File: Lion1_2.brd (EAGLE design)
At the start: 100 x 85.7 mm, 71 parts, among them IC1 MCP4822, IC2 MCP4822, IC3 MCP4822, IC4 REG1117, U7 2564-, U8 2564-

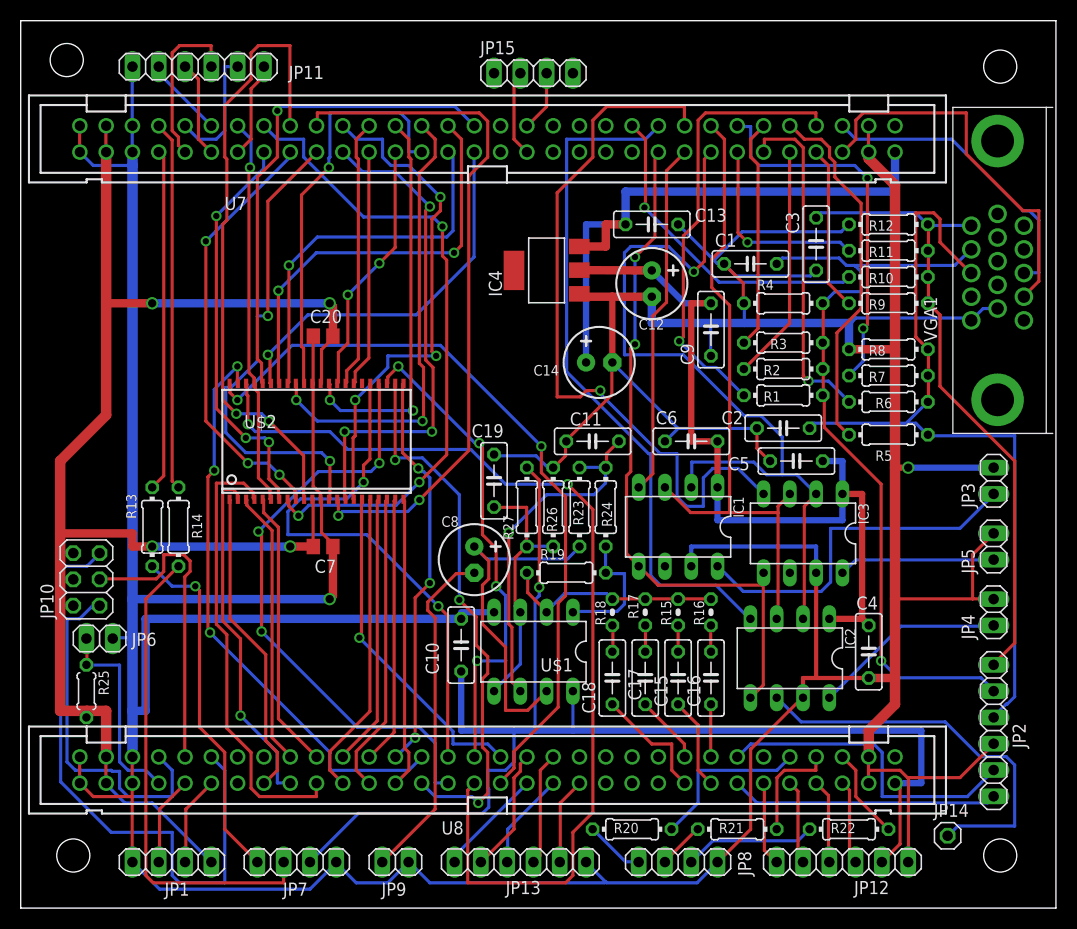
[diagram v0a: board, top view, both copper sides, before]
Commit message: v2
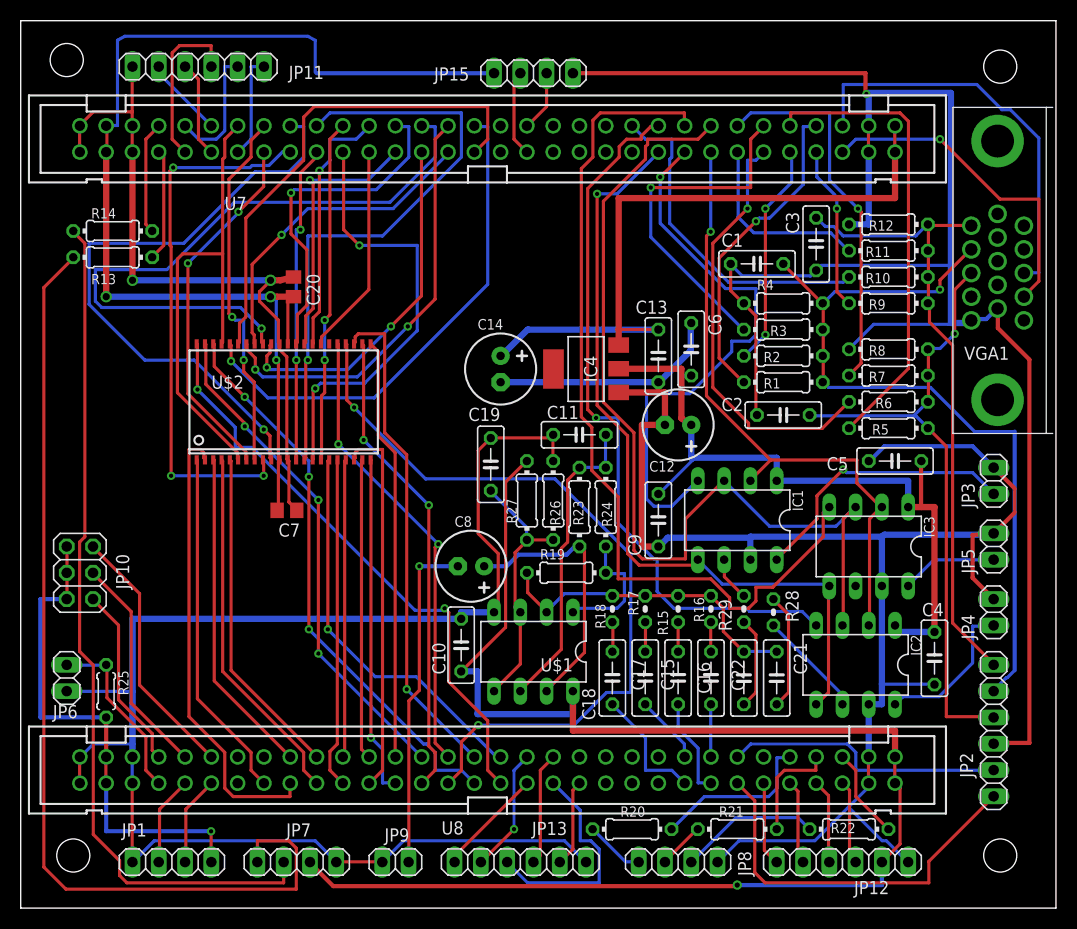
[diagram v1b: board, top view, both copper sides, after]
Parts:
- removed JP14: (no value), pinhead:1X01
- added C21, C22: 4.7uf, rcl:C050-025X075
- added R28, R29: (no value), SmartPrj:0204V
- C13: value 100nf -> (none)
- moved R14 29.3 mm to (8.89, 65.4), turned to 180 degrees
- moved R13 26.3 mm to (8.89, 62.9), turned to 180 degrees
- moved C9 19.1 mm to (61.6, 37.5)
- moved C12 13.9 mm to (63.5, 46.7), turned to 180 degrees
- moved C13 12.7 mm to (61.6, 53.3), turned to 90 degrees
- moved IC4 10.3 mm to (54.6, 52.1)
- moved C14 9.55 mm to (46.4, 52.1), turned to 270 degrees
- moved C5 9.52 mm to (84.5, 43.2)
- moved C6 8.89 mm to (64.8, 54.0), turned to 270 degrees
- moved IC3 6.48 mm to (81.9, 34.9)
- moved C4 6.38 mm to (88.3, 24.1)
- moved IC2 6.38 mm to (80.6, 23.5)
- moved IC1 5.75 mm to (69.2, 37.5)
- moved C20 5.55 mm to (26.4, 60.0), turned to 270 degrees
- moved U$2 4.96 mm to (25.4, 48.9)
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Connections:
- net N$24 renamed TX2
- net N$85 renamed RX2
- removed net 3V3: C20.2, C7.2, JP1.4, JP10.2, JP10.4, JP10.6, R25.2, U$2.11, U$2.33, U7.3, U7.4, U8.3, U8.4
- removed net GND: C1.1, C10.1, C11.2, C12.-, C13.1, C14.-, C19.1, C2.1, C20.1, C3.1, C4.1, C5.1, C6.1, C7.1, C9.1, IC1.7, IC2.7, IC3.7, IC4.1, JP1.1, JP11.1, JP12.1, JP13.1, JP2.4, JP3.2, JP4.2, JP5.2, JP6.2, JP7.4, JP8.4, JP9.2, R12.1, R26.1, R4.1, R8.1, U$1.4, U$2.12, U$2.34, U7.1, U7.2, U7.5, U7.6, U7.61, U7.62, U8.1, U8.2, U8.5, U8.6, U8.61, U8.62, VGA1.10, VGA1.5
- removed net N$70: U8.64
- new net 3V3_7: C20.2, C7.2, JP15.1, U$2.11, U$2.33, U7.3, U7.4
- new net 3V3_8: JP1.4, JP10.2, JP10.4, JP10.6, R25.2, U8.3, U8.4
- new net ADD: C21.1, C22.1, R15.2, R16.2, R17.2, R18.2, R19.1, U$1.2
- new net GND7_61: C1.1, C2.1, C3.1, JP15.4, JP2.4, R12.1, R4.1, R8.1, U7.61, U7.62, VGA1.10, VGA1.5
- new net GND8_1: C10.1, C11.2, C19.1, JP1.1, JP13.1, JP6.2, JP7.4, JP9.2, R26.1, U$1.4, U8.1, U8.2, U8.5, U8.6
- new net GND_: C12.-, C13.1, C14.-, C4.1, C5.1, C6.1, C9.1, IC1.7, IC2.7, IC3.7, IC4.1, JP12.1, JP3.2, JP4.2, JP5.2, JP8.4, U8.61, U8.62
- new net GND_1: C20.1, C7.1, JP11.1, U$2.12, U$2.34, U7.1, U7.2, U7.5, U7.6
- new net N$25: C22.2, R29.1
- new net N$26: IC1.6, R29.2
- net 5V: now also U8.64
- net 5V_2: now also U7.64
- net N$2: now also R28.2; no longer JP14.1
- net N$9: now also C21.2, R28.1; no longer R15.2, R16.2, R17.2, R18.2, R19.1, U$1.2
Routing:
- net GND: track 559.1 -> 0.00 mm, vias 2 -> 0
- net GND7_61: track 0.00 -> 176.1 mm, vias 0 -> 1
- net GND_: track 0.00 -> 168.4 mm
- net 3V3: track 148.1 -> 0.00 mm, vias 4 -> 0
- net GND8_1: track 0.00 -> 148.0 mm
- net 3V3_7: track 0.00 -> 110.0 mm, vias 0 -> 3
- net GND_1: track 0.00 -> 68.6 mm, vias 0 -> 2
- net N$12: track 34.1 -> 95.4 mm, vias 1 -> 0
- net 3V3_8: track 0.00 -> 49.6 mm, vias 0 -> 1
- net A16: track 97.2 -> 54.6 mm, vias 2 -> 3
- net N$13: track 46.8 -> 82.7 mm
- net INT: track 60.2 -> 25.0 mm
- net ADD: track 0.00 -> 31.3 mm
- net D1: track 63.3 -> 35.2 mm, vias 3 -> 2
- net N$2: track 38.4 -> 10.4 mm
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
